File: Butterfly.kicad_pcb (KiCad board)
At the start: 2 copper layers, 93.1 x 65.5 mm, 28 parts, among them J1 Conn_02x03_Odd_Even, J2 USB_A, U1 ATTINY85-20PU

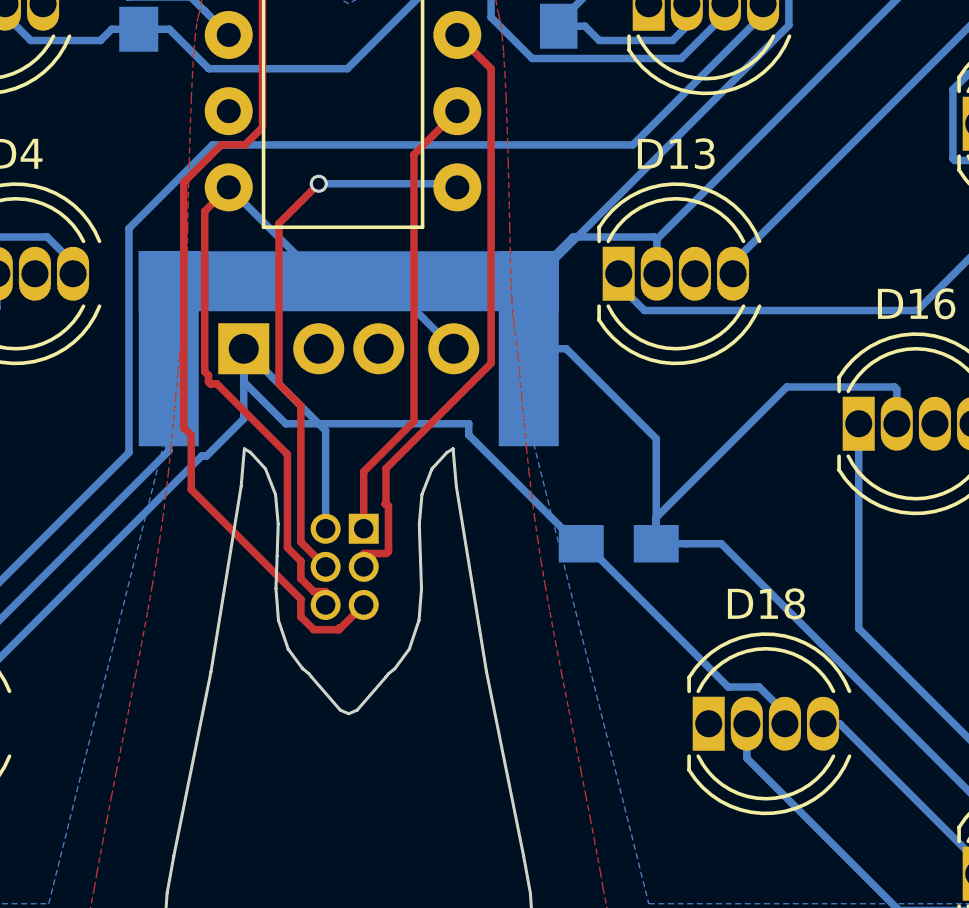
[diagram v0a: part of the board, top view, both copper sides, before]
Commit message: I think I got everything to fit.
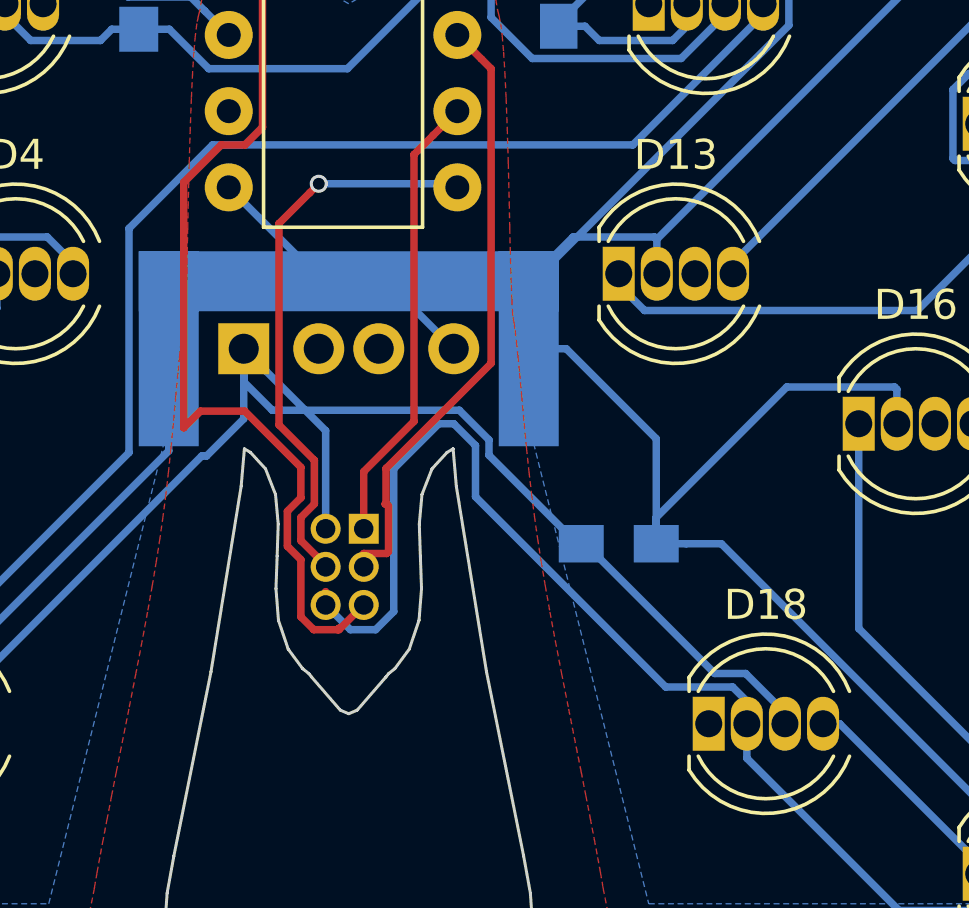
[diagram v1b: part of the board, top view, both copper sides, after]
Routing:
- net GND: track 391.6 -> 401.3 mm
- net Net-(J1-Pad5): track 32.0 -> 34.4 mm
